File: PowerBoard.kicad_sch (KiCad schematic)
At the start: 94 parts, among them IC1 LTC7004HMSE#PBF, IC2 LTC7004HMSE#PBF, IC3 LTC7004HMSE#PBF, J1 XT90, J10 DEAN_T, J11 DEAN_T, J12 DEAN_T, J13 DEAN_T, J14 DEAN_T, J15 DEAN_T, J16 XT60, J17 XT60, J18 XT60, J19 XT60, J2 DEAN_T, J20 XT60, J21 XT60, J22 XT30, J23 XT30, J24 XT30, J25 XT30, J26 XT30, J27 XT30, J28 XT90, J29 XT30, J3 XT60, J30 XT30, J31 XT30, J32 Conn_01x02, J4 XT30, J5 XT90, J6 XT90, J7 XT90, J8 XT90, J9 XT90, Q1 IRFS7437TRLPBF, Q2 IRFS7437TRLPBF, Q3 IRFS7437TRLPBF, U1 Pico, U2 LM317_TO-220

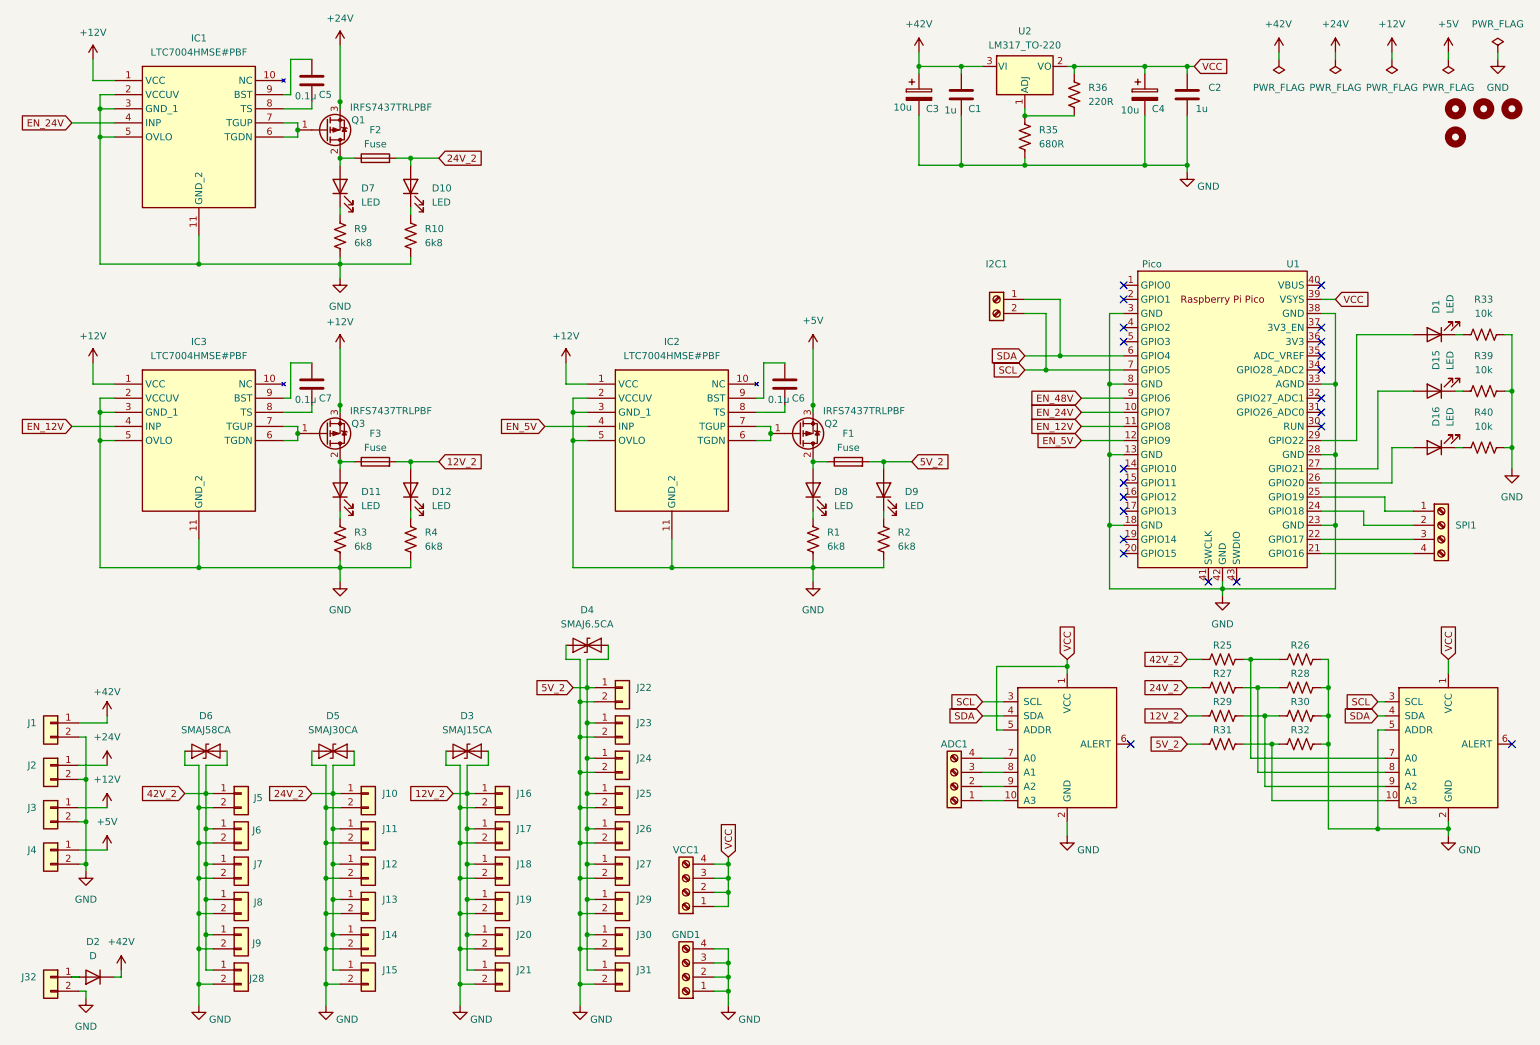
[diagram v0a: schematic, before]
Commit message: iterate the layoutL
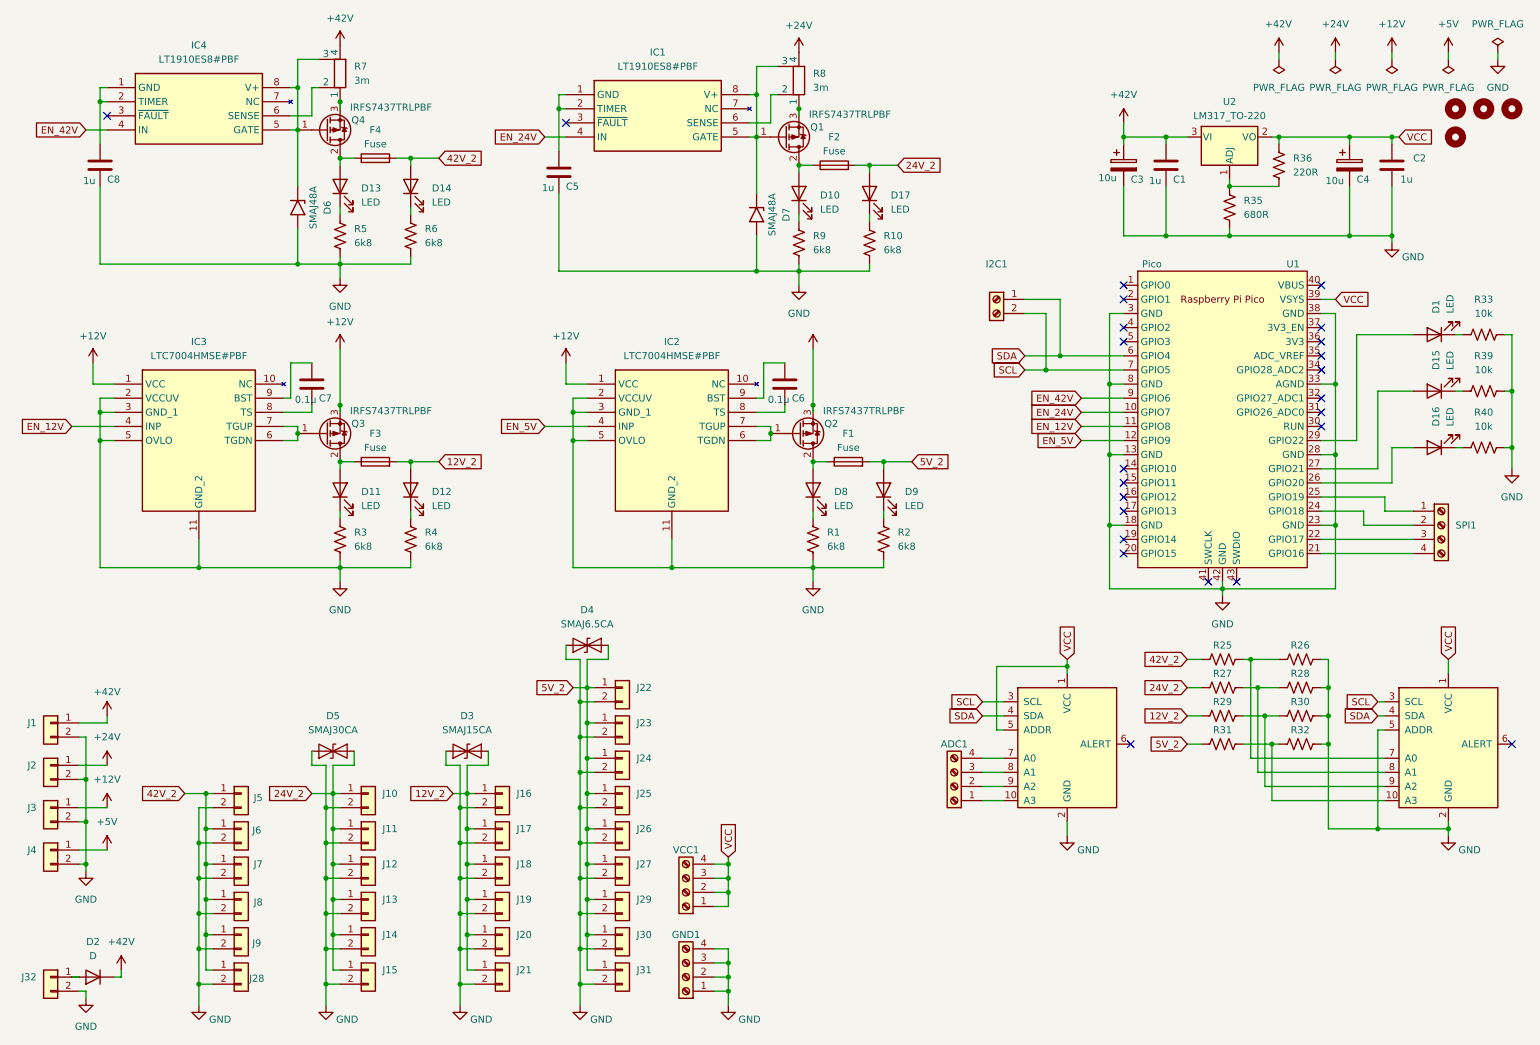
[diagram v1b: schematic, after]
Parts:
- removed D6: SMAJ58CA, Diode_SMD:D_SMA, symbol Diode:SMAJ58CA
- removed D7: LED, Diode_SMD:D_1206_3216Metric, symbol Device:LED
- removed IC1: LTC7004HMSE#PBF, SOP50P490X110-11N, symbol SamacSys_Parts:LTC7004HMSE#PBF
- added C8: 1u, Capacitor_SMD:C_1206_3216Metric, symbol Device:C
- added D13, D14, D17: LED, Diode_SMD:D_1206_3216Metric, symbol Device:LED
- added D6, D7: SMAJ48A, Diode_SMD:D_SMA, symbol Diode:SMAJ48A
- added F4: Fuse, Fuse:Fuse_Blade_ATO_directSolder, symbol Device:Fuse
- added IC1, IC4: LT1910ES8#PBF, SOIC127P599X175-8N, symbol SamacSys_Parts:LT1910ES8#PBF
- added Q4: IRFS7437TRLPBF, Package_TO_SOT_SMD:TO-263-2, symbol Transistor_FET:IRF9540N
- added R5, R6: 6k8, Resistor_SMD:R_1206_3216Metric, symbol Device:R_US
- added R7, R8: 3m, Resistor_SMD:R_Shunt_Isabellenhuette_BVR4026, symbol Device:R_Shunt
- C5: value 0.1u -> 1u
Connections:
- net +24V: now also R8.4; no longer Q1.3 (S)
- net +42V: now also R7.4
- net 24V_2: now also D17.2 (A); no longer D10.2 (A)
- net 42V_2: now also D14.2 (A), F4.2
- net EN_24V: now also IC1.4 (IN)
- net GND: now also C5.2, C8.2, D6.2 (A2), D7.2 (A2), R5.2, R6.2
- net at Q1.1 (G): now also D7.1 (A1), IC1.5 (GATE), IC1.8 (V+), R8.3
- net at C5.1: now also IC1.1 (GND), IC1.2 (TIMER)
- net at F2.1, Q1.2 (D): now also D10.2 (A)
- net at R9.1: now also D10.1 (K)
- net at R10.1: now also D17.1 (K); no longer D10.1 (K)
- net EN_48V renamed EN_42V
- net EN_42V: now also IC4.4 (IN)
- new net: Q4.3 (S), R7.1
- new net: IC4.6 (SENSE), R7.2
- new net: D6.1 (A1), IC4.5 (GATE), IC4.8 (V+), Q4.1 (G), R7.3
- new net: D14.1 (K), R6.1
- new net: D13.2 (A), F4.1, Q4.2 (D)
- new net: IC1.6 (SENSE), R8.2
- new net: C8.1, IC4.1 (GND), IC4.2 (TIMER)
- new net: Q1.3 (S), R8.1
- new net: D13.1 (K), R5.1
- no-connect marks 22 -> 24
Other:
- moved on the sheet: C1, C2, C3, C4, R35, R36, U2
